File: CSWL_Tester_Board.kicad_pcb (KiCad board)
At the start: 2 copper layers, 160 x 170 mm, 214 parts, among them J1 Conn_02x10_Odd_Even, J2 Conn_01x03, J3 Conn_02x10_Odd_Even, J4 IDC 2.54mm, Q1 2N7002LT1G, Q2 2N7002LT1G, Q3 2N7002LT1G, Q4 2N7002LT1G, Q5 2N7002LT1G, Q6 2N7002LT1G, Q7 2N7002LT1G, Q8 2N7002LT1G, Q9 2N7002LT1G, U1 CD74HC4067M, U10 sn74hc595, U11 sn74hc595, U12 sn74hc595, U13 sn74hc595, U14 TCS3200, U15 TCS3200, U16 TCS3200, U17 TCS3200, U18 TCS3200, U19 TCS3200, U2 CD74HC4067M, U20 TCS3200, U21 TCS3200, U22 TCS3200, U23 TCS3200, U24 TCS3200, U25 TCS3200, U26 SN74HC151DR, U27 MCP1700T-3302E_TT, U28 SN74HC151DR, U29 74HC4016, U3 MCP1700T-3302E_TT, U4 sn74hc595, U5 sn74hc595, U6 sn74hc595, U7 STM32F103C8Tx, U8 sn74hc595, U9 sn74hc595, Y1 Crystal_GND24

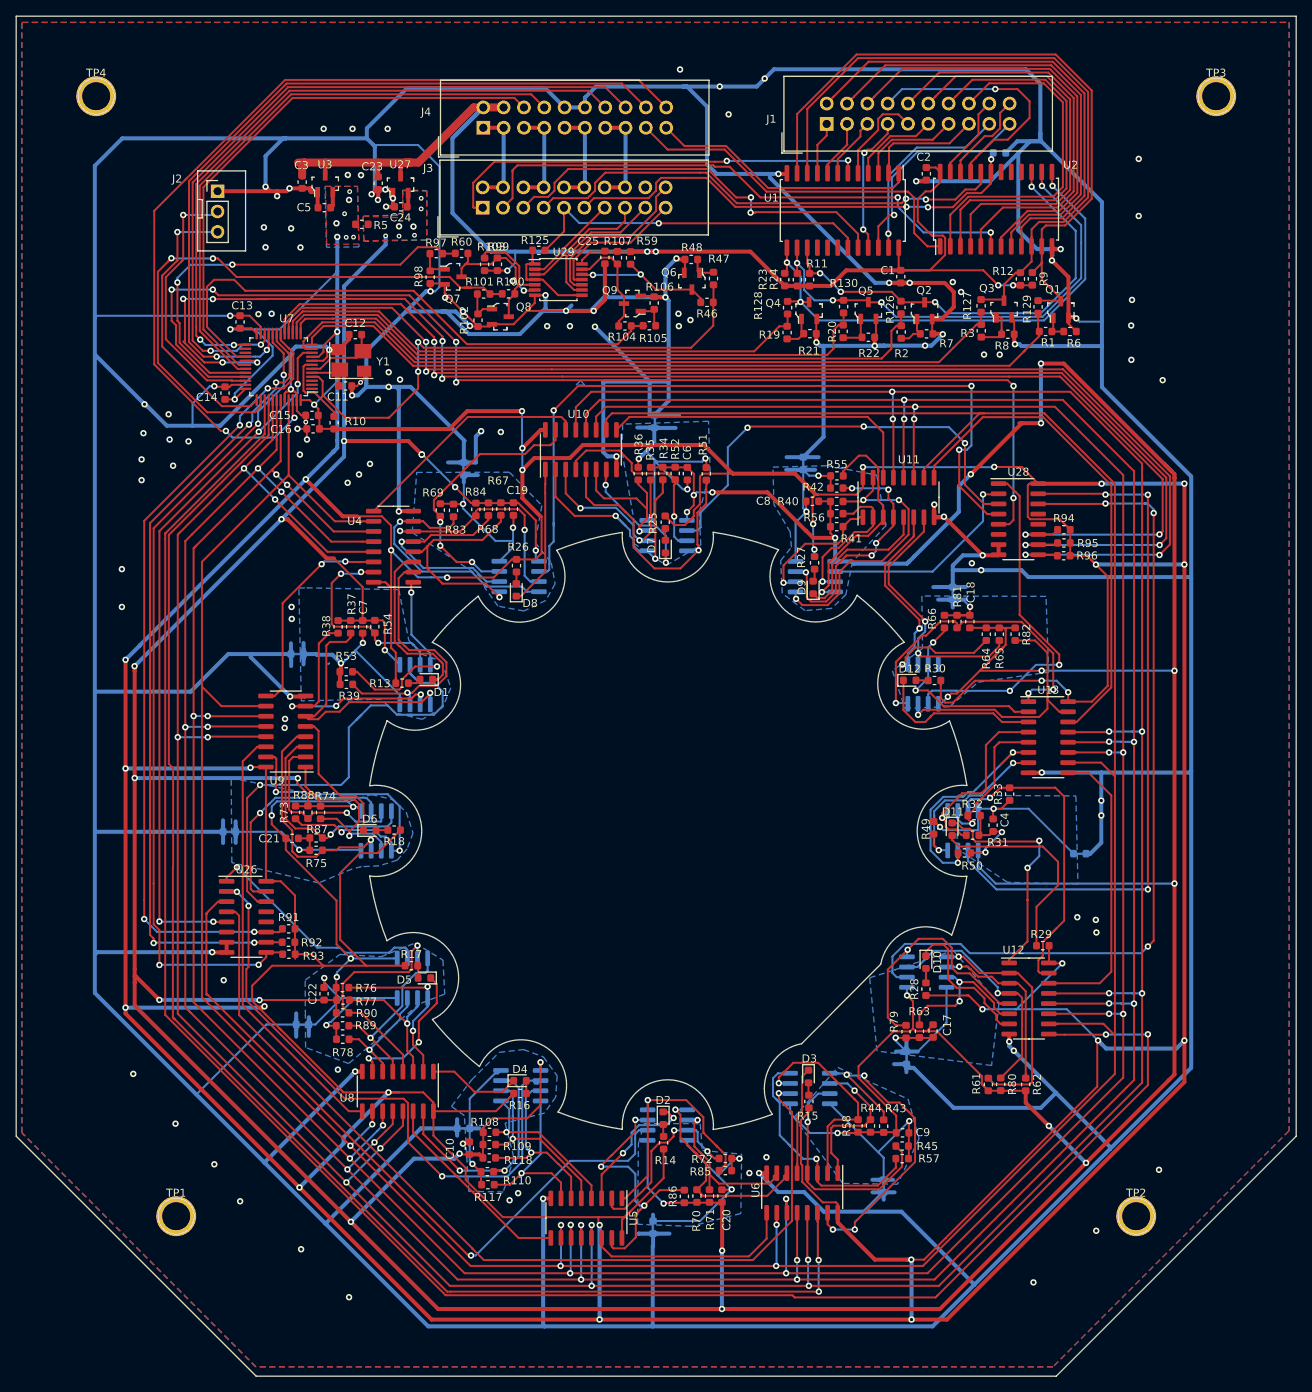
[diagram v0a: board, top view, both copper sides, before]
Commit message: Ruan: add treatdrop
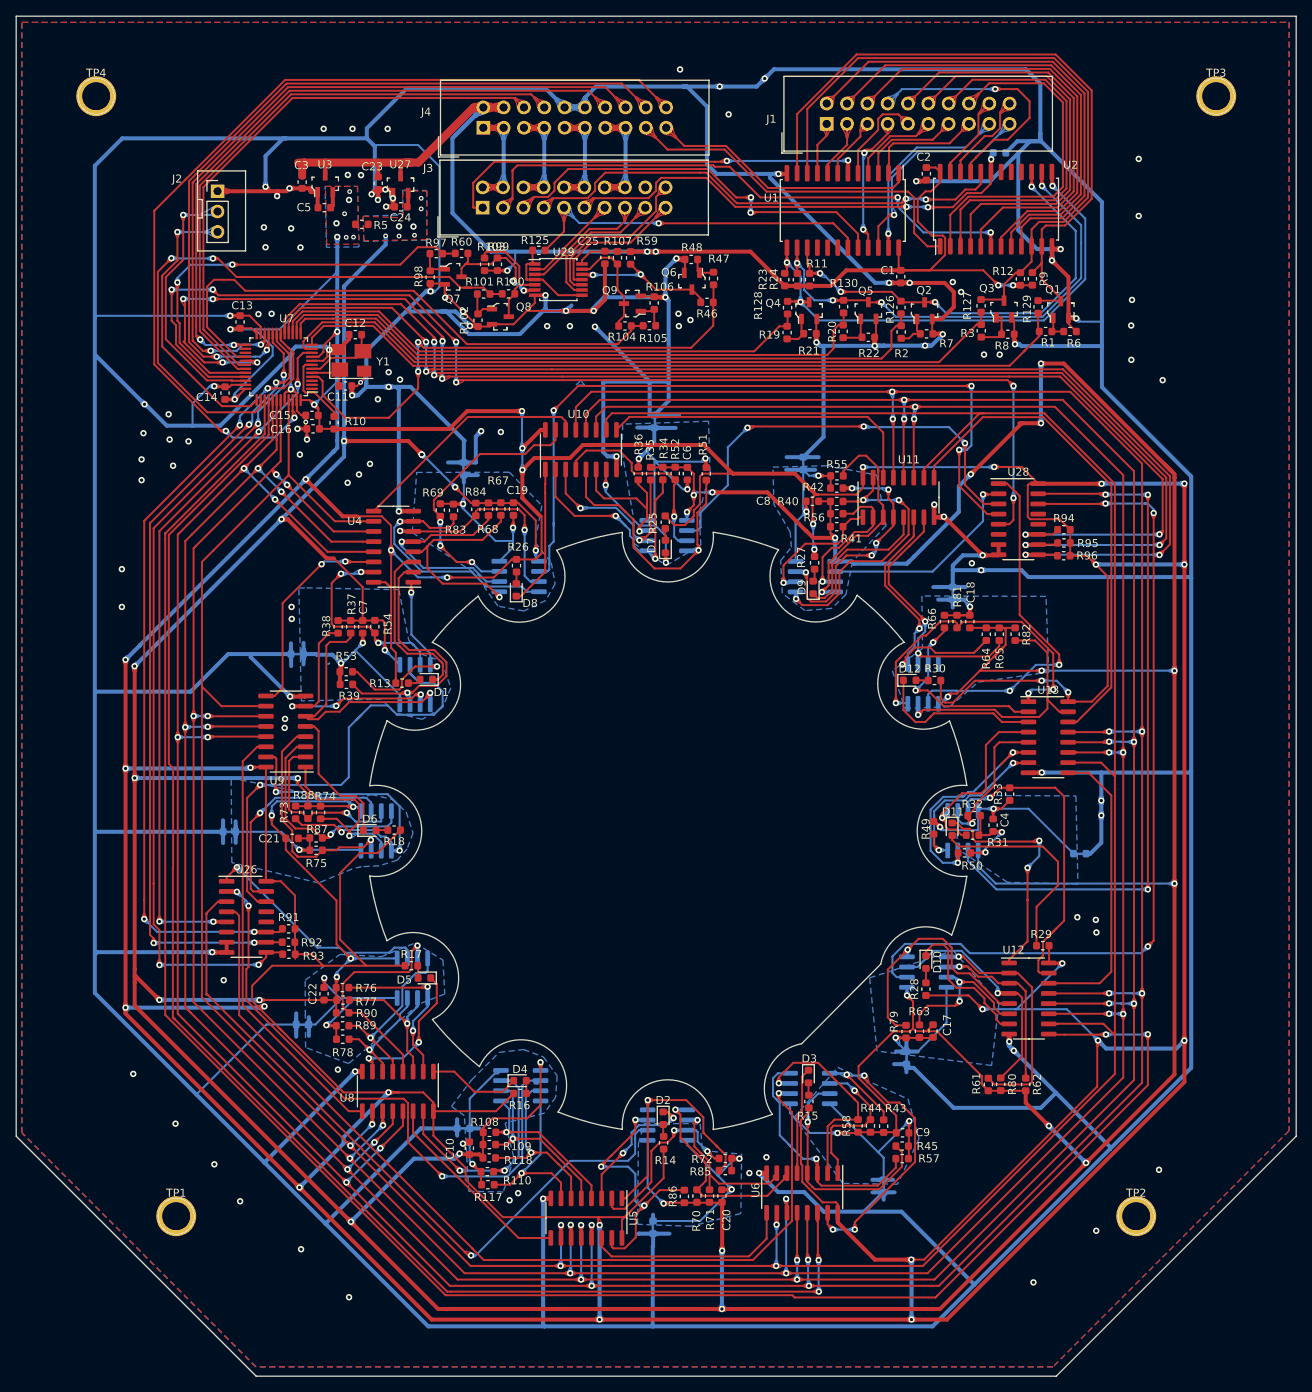
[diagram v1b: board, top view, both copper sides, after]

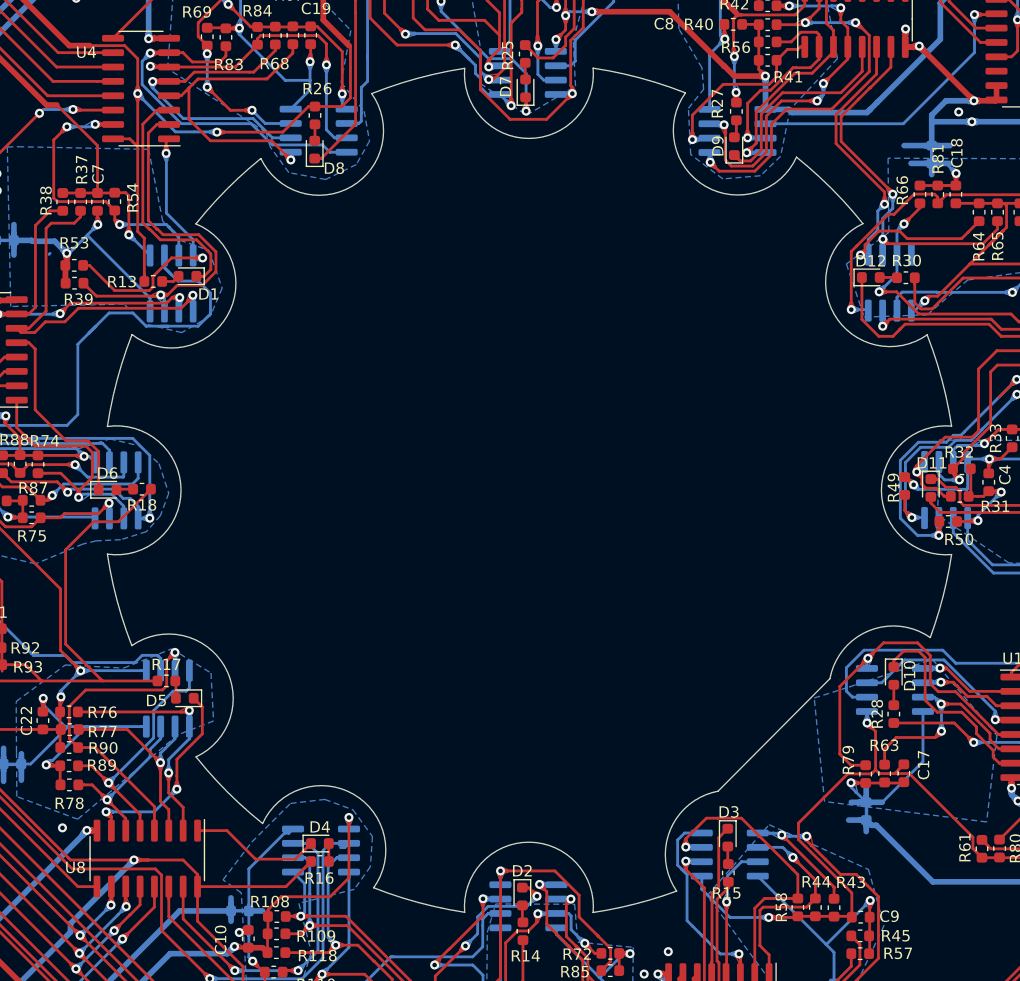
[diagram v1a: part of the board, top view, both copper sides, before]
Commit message: Ruan: modify shape
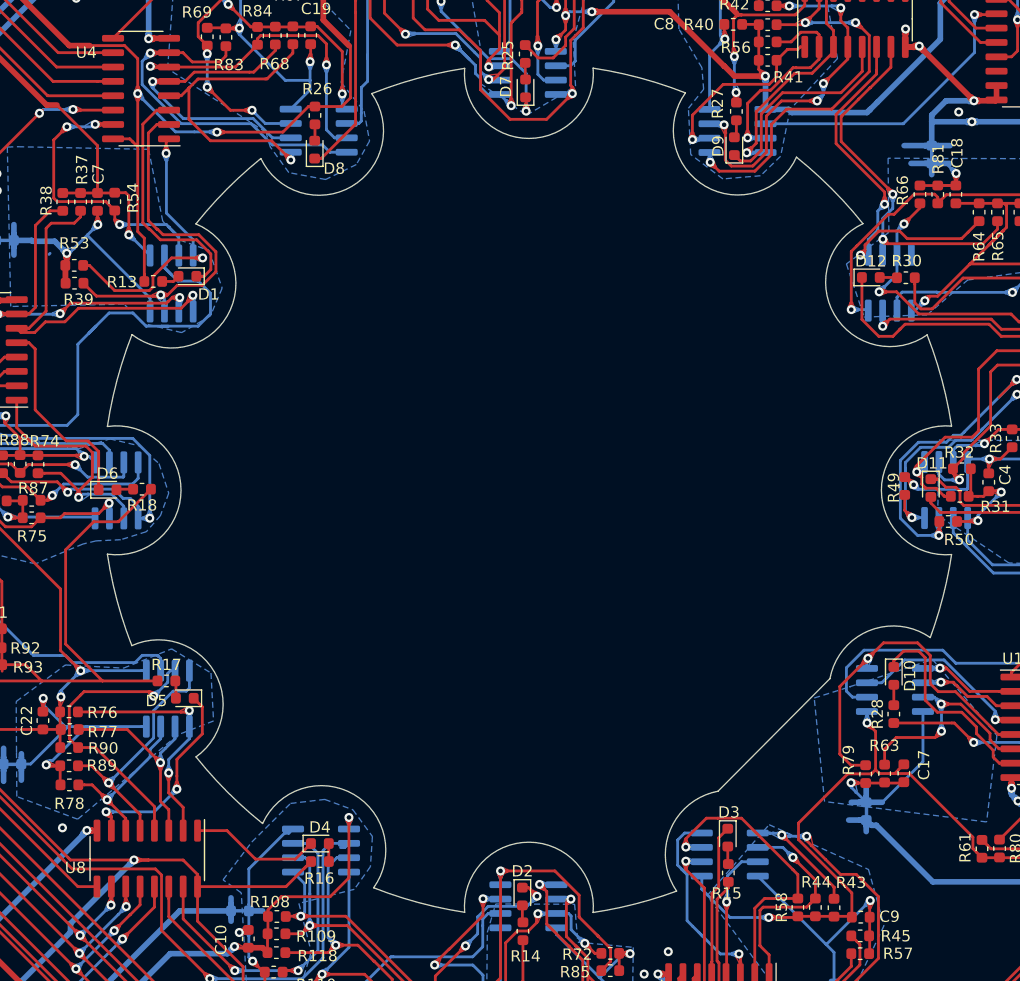
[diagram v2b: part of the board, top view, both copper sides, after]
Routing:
- net /LED4_S2: track 29.2 -> 26.5 mm
